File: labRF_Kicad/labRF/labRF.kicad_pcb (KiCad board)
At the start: 2 copper layers, 71 x 78 mm, 1 part, among them U1 ATmega328-P

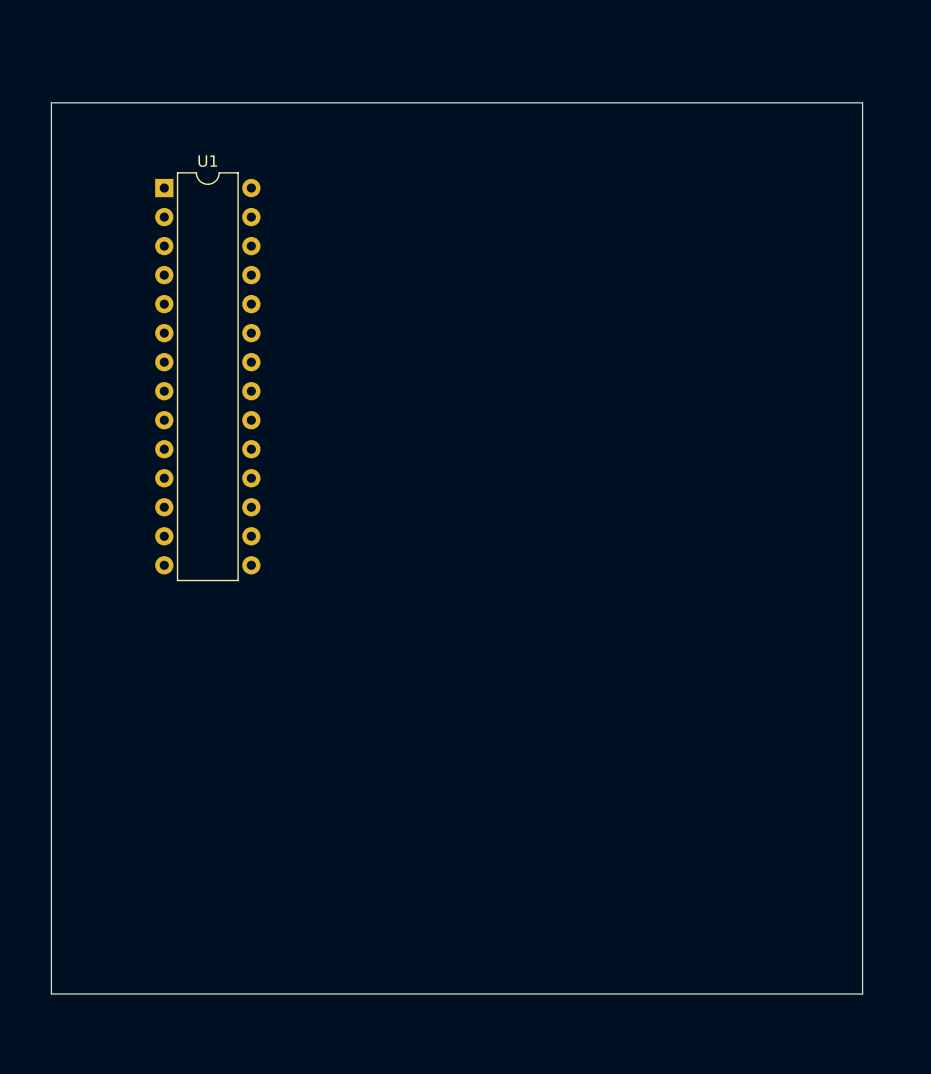
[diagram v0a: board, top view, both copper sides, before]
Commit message: Finieshed PCB Design
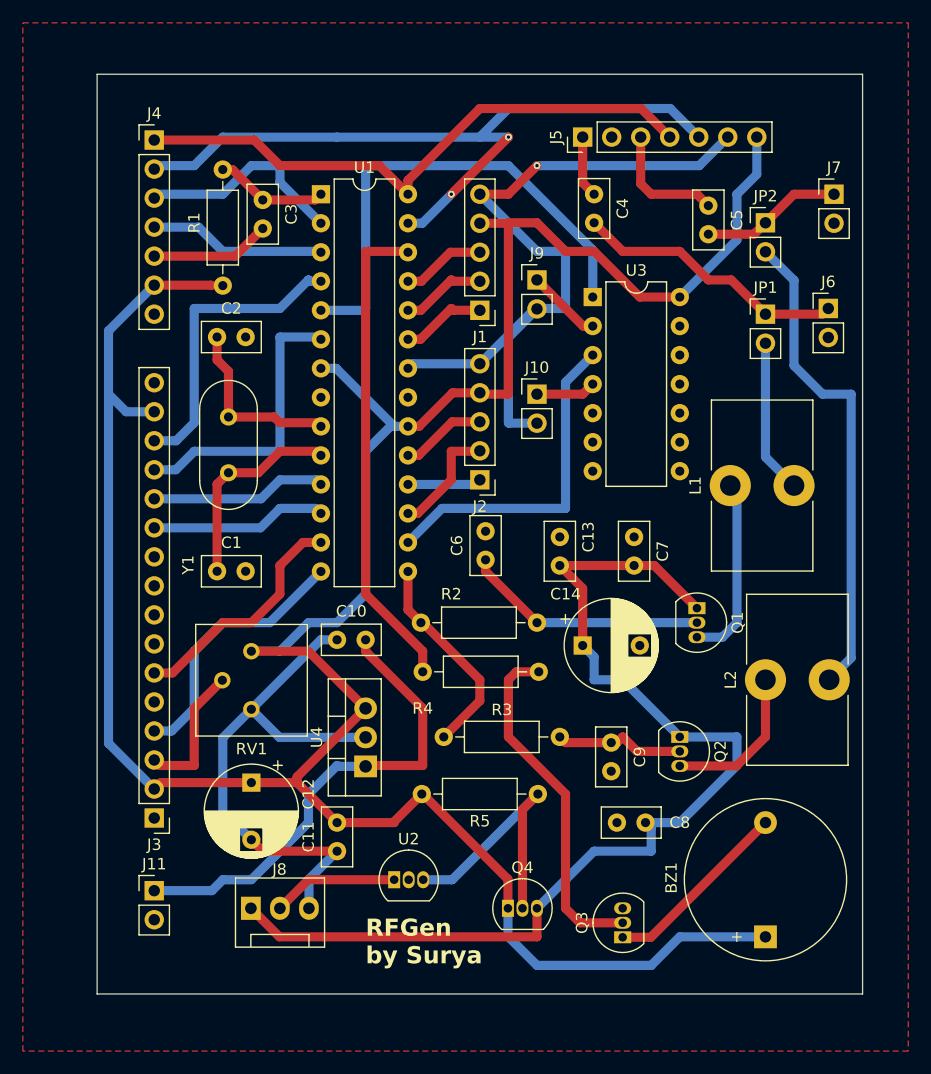
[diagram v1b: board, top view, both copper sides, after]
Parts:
- added BZ1: Buzzer, Buzzer_Beeper:Buzzer_D14mm_H7mm_P10mm, F.Cu at (100.0, 102.5)
- added C1: 22p, Capacitor_THT:C_Disc_D5.0mm_W2.5mm_P2.50mm, F.Cu at (52.0, 70.5)
- added C10: 10n, Capacitor_THT:C_Disc_D5.0mm_W2.5mm_P2.50mm, F.Cu at (62.5, 76.5)
- added C11: 100n, Capacitor_THT:C_Disc_D5.0mm_W2.5mm_P2.50mm, F.Cu at (62.5, 95.0)
- added C12: 100u, Capacitor_THT:CP_Radial_D8.0mm_P5.00mm, F.Cu at (55.0, 89.0)
- added C13: 100n, Capacitor_THT:C_Disc_D5.0mm_W2.5mm_P2.50mm, F.Cu at (82.0, 67.5)
- added C14: 100u, Capacitor_THT:CP_Radial_D8.0mm_P5.00mm, F.Cu at (84.0, 77.0)
- added C2: 22p, Capacitor_THT:C_Disc_D5.0mm_W2.5mm_P2.50mm, F.Cu at (52.0, 50.0)
- added C3: 100n, Capacitor_THT:C_Disc_D5.0mm_W2.5mm_P2.50mm, F.Cu at (56.0, 38.0)
- added C4: 100n, Capacitor_THT:C_Disc_D5.0mm_W2.5mm_P2.50mm, F.Cu at (85.0, 37.5)
- added C5: 100n, Capacitor_THT:C_Disc_D5.0mm_W2.5mm_P2.50mm, F.Cu at (95.0, 38.5)
- added C6: 10n, Capacitor_THT:C_Disc_D5.0mm_W2.5mm_P2.50mm, F.Cu at (75.5, 69.5)
- added C7: 10n, Capacitor_THT:C_Disc_D5.0mm_W2.5mm_P2.50mm, F.Cu at (88.5, 67.5)
- added C8: 10n, Capacitor_THT:C_Disc_D5.0mm_W2.5mm_P2.50mm, F.Cu at (87.0, 92.5)
- added C9: 10n, Capacitor_THT:C_Disc_D5.0mm_W2.5mm_P2.50mm, F.Cu at (86.5, 85.5)
- added J1: select_rotary, Connector_PinHeader_2.54mm:PinHeader_1x05_P2.54mm_Vertical, F.Cu at (75.0, 47.7)
- added J10: pwmC, Connector_PinHeader_2.54mm:PinHeader_1x02_P2.54mm_Vertical, F.Cu at (80.0, 55.0)
- added J11: pwrIn, Connector_PinHeader_2.54mm:PinHeader_1x02_P2.54mm_Vertical, F.Cu at (46.5, 98.5)
- added J2: mode_rotary, Connector_PinHeader_2.54mm:PinHeader_1x05_P2.54mm_Vertical, F.Cu at (75.0, 62.5)
- added J3: lcd_socket, Connector_PinHeader_2.54mm:PinHeader_1x16_P2.54mm_Vertical, F.Cu at (46.5, 92.1)
- added J4: comms, Connector_PinHeader_2.54mm:PinHeader_1x07_P2.54mm_Vertical, F.Cu at (46.5, 32.8)
- added J5: si5351, Connector_PinHeader_2.54mm:PinHeader_1x07_P2.54mm_Vertical, F.Cu at (84.0, 32.5)
- added J6: clk0, Connector_PinHeader_2.54mm:PinHeader_1x02_P2.54mm_Vertical, F.Cu at (105.5, 47.5)
- added J7: clk2, Connector_PinHeader_2.54mm:PinHeader_1x02_P2.54mm_Vertical, F.Cu at (106.0, 37.5)
- added J8: bias_pot, Connector:FanPinHeader_1x03_P2.54mm_Vertical, F.Cu at (55.0, 100.0)
- added J9: pwmD, Connector_PinHeader_2.54mm:PinHeader_1x02_P2.54mm_Vertical, F.Cu at (80.0, 45.0)
- added JP1: Jumper_2_Open, Connector_PinHeader_2.54mm:PinHeader_1x02_P2.54mm_Vertical, F.Cu at (100.0, 48.0)
- added JP2: Jumper_2_Open, Connector_PinHeader_2.54mm:PinHeader_1x02_P2.54mm_Vertical, F.Cu at (100.0, 40.0)
- added L1: 100u, Inductor_THT:L_Toroid_Vertical_L14.7mm_W8.6mm_P5.58mm_Pulse_KM-1, F.Cu at (96.9, 63.0)
- added L2: 100u, Inductor_THT:L_Toroid_Vertical_L14.7mm_W8.6mm_P5.58mm_Pulse_KM-1, F.Cu at (100.0, 80.0)
- added Q1: BC547, Package_TO_SOT_THT:TO-92_Inline, F.Cu at (94.0, 73.7)
- added Q2: BC547, Package_TO_SOT_THT:TO-92_Inline, F.Cu at (92.5, 85.0)
- added Q3: BC547, Package_TO_SOT_THT:TO-92_Inline, F.Cu at (87.5, 102.5)
- added Q4: BC547, Package_TO_SOT_THT:TO-92_Inline, F.Cu at (77.5, 100.0)
- added R1: 10k, Resistor_THT:R_Axial_DIN0207_L6.3mm_D2.5mm_P10.16mm_Horizontal, F.Cu at (52.5, 35.3)
- added R2: 10k, Resistor_THT:R_Axial_DIN0207_L6.3mm_D2.5mm_P10.16mm_Horizontal, F.Cu at (69.8, 75.0)
- added R3: 10k, Resistor_THT:R_Axial_DIN0207_L6.3mm_D2.5mm_P10.16mm_Horizontal, F.Cu at (71.8, 85.0)
- added R4: 2.2k, Resistor_THT:R_Axial_DIN0207_L6.3mm_D2.5mm_P10.16mm_Horizontal, F.Cu at (70.0, 79.3)
- added R5: 1k, Resistor_THT:R_Axial_DIN0207_L6.3mm_D2.5mm_P10.16mm_Horizontal, F.Cu at (80.1, 90.0)
- added RV1: R_Potentiometer, Potentiometer_THT:Potentiometer_Bourns_3386P_Vertical, F.Cu at (55.0, 77.5)
- added U2: TL431LP, Package_TO_SOT_THT:TO-92_Inline, F.Cu at (67.5, 97.5)
- added U3: 74HC04, Package_DIP:DIP-14_W7.62mm, F.Cu at (84.9, 46.5)
- added U4: L7805, Package_TO_SOT_THT:TO-220-3_Vertical, F.Cu at (65.0, 87.6)
- added Y1: 20Mhz, Crystal:Crystal_HC49-U_Vertical, F.Cu at (53.0, 61.9)
- moved U1 13.7 mm to (61.1, 37.5)
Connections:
- net Net-(U1-GND-Pad22) renamed GND
- U1 pad 1: unconnected-(U1-~{RESET}/PC6-Pad1) -> Net-(U1-~{RESET}/PC6)
- U1 pad 10: unconnected-(U1-XTAL2/PB7-Pad10) -> Net-(U1-XTAL2/PB7)
- U1 pad 11: unconnected-(U1-PD5-Pad11) -> lcd_D5
- U1 pad 12: unconnected-(U1-PD6-Pad12) -> lcd_D4
- U1 pad 13: unconnected-(U1-PD7-Pad13) -> lcd_enb
- U1 pad 14: unconnected-(U1-PB0-Pad14) -> lcd_rs
- U1 pad 15: unconnected-(U1-PB1-Pad15) -> bias
- U1 pad 16: unconnected-(U1-PB2-Pad16) -> chanc
- U1 pad 17: unconnected-(U1-PB3-Pad17) -> rotm_dt
- U1 pad 18: unconnected-(U1-PB4-Pad18) -> rotm_clk
- U1 pad 19: unconnected-(U1-PB5-Pad19) -> rotm_sw
- U1 pad 2: unconnected-(U1-PD0-Pad2) -> rx
- U1 pad 20: unconnected-(U1-AVCC-Pad20) -> +5V
- U1 pad 23: unconnected-(U1-PC0-Pad23) -> rots_clk
- U1 pad 24: unconnected-(U1-PC1-Pad24) -> rots_dt
- U1 pad 25: unconnected-(U1-PC2-Pad25) -> rots_sw
- U1 pad 26: unconnected-(U1-PC3-Pad26) -> buzz
- U1 pad 27: unconnected-(U1-PC4-Pad27) -> sda
- U1 pad 28: unconnected-(U1-PC5-Pad28) -> scl
- U1 pad 3: unconnected-(U1-PD1-Pad3) -> tx
- U1 pad 4: unconnected-(U1-PD2-Pad4) -> lcd_D7
- U1 pad 5: unconnected-(U1-PD3-Pad5) -> chand
- U1 pad 6: unconnected-(U1-PD4-Pad6) -> lcd_D6
- U1 pad 7: unconnected-(U1-VCC-Pad7) -> +5V
- U1 pad 9: unconnected-(U1-XTAL1/PB6-Pad9) -> Net-(U1-XTAL1/PB6)
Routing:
- net +5V: track 0.00 -> 244.3 mm
- net GND: track 0.00 -> 116.9 mm, vias 0 -> 1
- net Net-(J8-Pin_1): track 0.00 -> 95.3 mm
- net sda: track 0.00 -> 65.3 mm, vias 0 -> 2
- net scl: track 0.00 -> 51.9 mm
- net chand: track 0.00 -> 43.5 mm
- net Net-(JP2-B): track 0.00 -> 42.8 mm
- net Net-(J11-Pin_1): track 0.00 -> 42.6 mm
- net buzz: track 0.00 -> 42.6 mm
- net Net-(Q3-B): track 0.00 -> 30.5 mm
- net chanc: track 0.00 -> 29.4 mm
- net lcd_D7: track 0.00 -> 26.3 mm
- net lcd_D6: track 0.00 -> 25.3 mm
- net Net-(J6-Pin_1): track 0.00 -> 24.0 mm
- net Net-(Q4-B): track 0.00 -> 23.7 mm
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- added copper zone on F.Cu, net GND
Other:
- board size 71 x 78 mm -> 67 x 80.5 mm
- board text added: "RFGen by Surya"
